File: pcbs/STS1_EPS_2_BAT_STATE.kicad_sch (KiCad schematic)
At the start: 10 parts, among them U4 MIC841H, U5 MIC841L

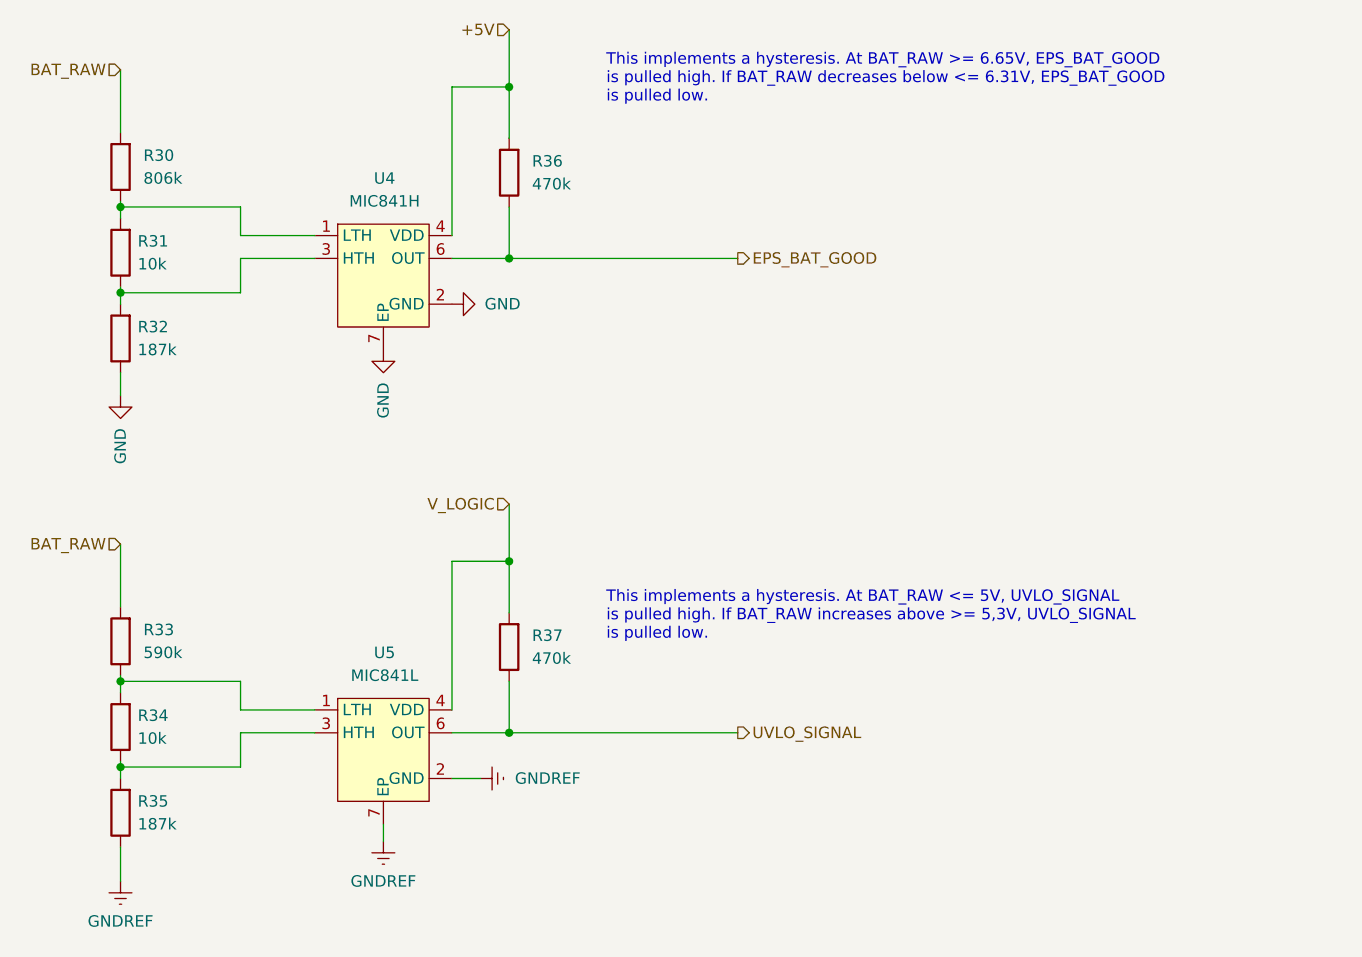
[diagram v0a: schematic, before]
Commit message: Intermediate commit.
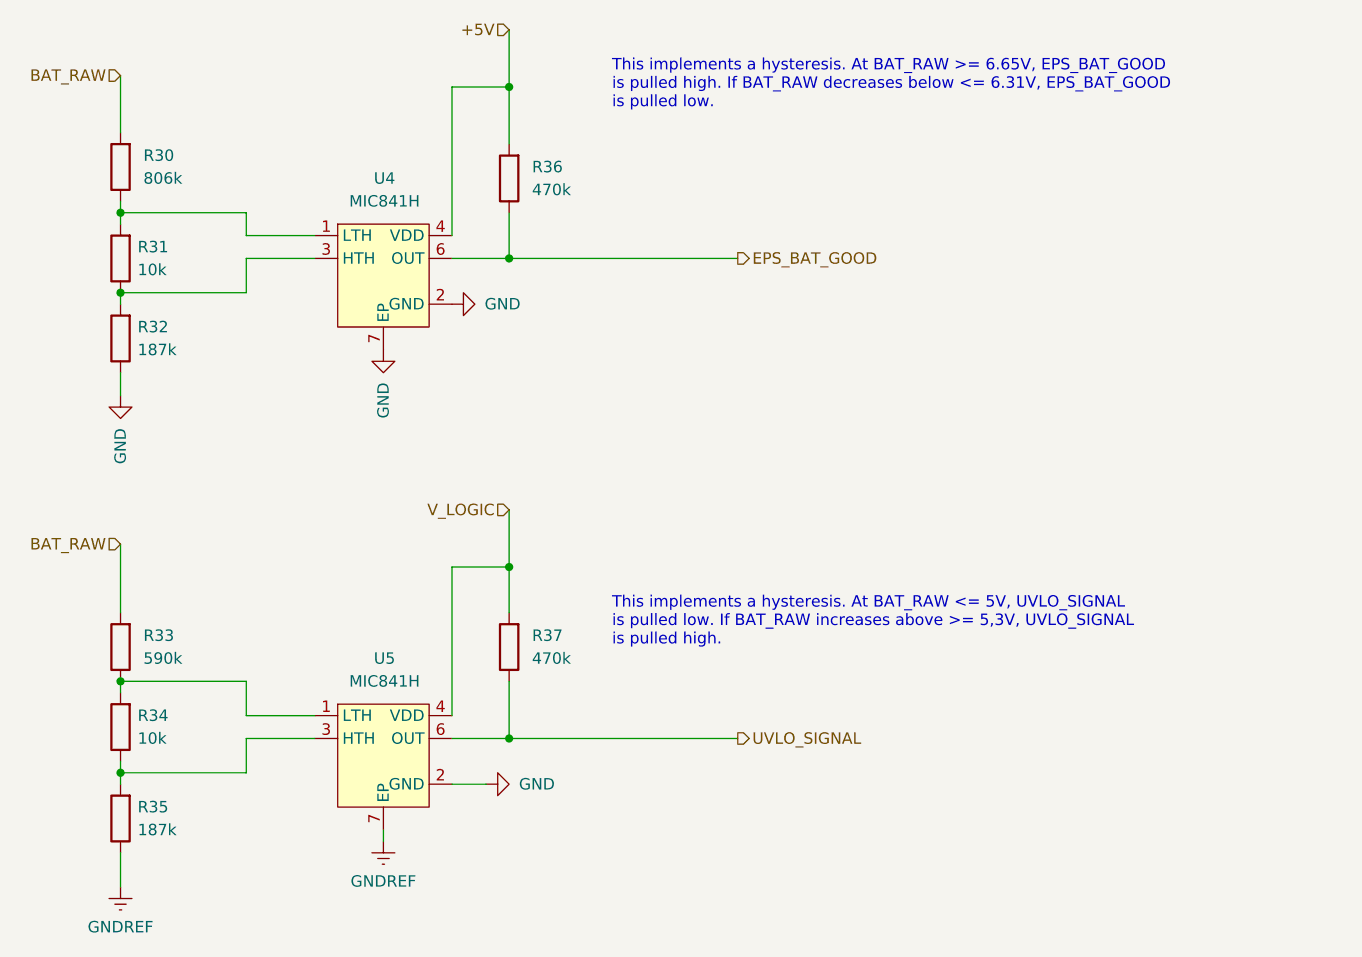
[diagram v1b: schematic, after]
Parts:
- U5: value MIC841L -> MIC841H
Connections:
- net GND: now also U5.2 (GND)
- net GNDREF: no longer U5.2 (GND)
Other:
- note added: "This implements a hysteresis. At BAT_RAW <= 5V, UVLO_SIGNAL is pulled low. If BAT_RAW increases above >= 5,3V, UVLO_SIGNAL is pulled high."
- note removed: "This implements a hysteresis. At BAT_RAW <= 5V, UVLO_SIGNAL is pulled high. If BAT_RAW increases above >= 5,3V, UVLO_SIGNAL is pulled low."
- moved on the sheet: R31, R33, R35, R36, U5
